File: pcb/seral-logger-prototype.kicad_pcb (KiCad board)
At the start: 2 copper layers, 108 x 23 mm, 49 parts, among them J1 Conn_ARM_JTAG_SWD_10, J2 Conn_01x04_Female, J3 Conn_01x04_Female, SW1 Rotary_Encoder_Switch_RGB, SW2 SW_SPST, U1 STM32G070KBT6, U2 74LVC3G17, U3 TLV70228_SOT23-5, U4 sn74lv1t34, U5 TLV61046ADB, U6 sn74lv1t34

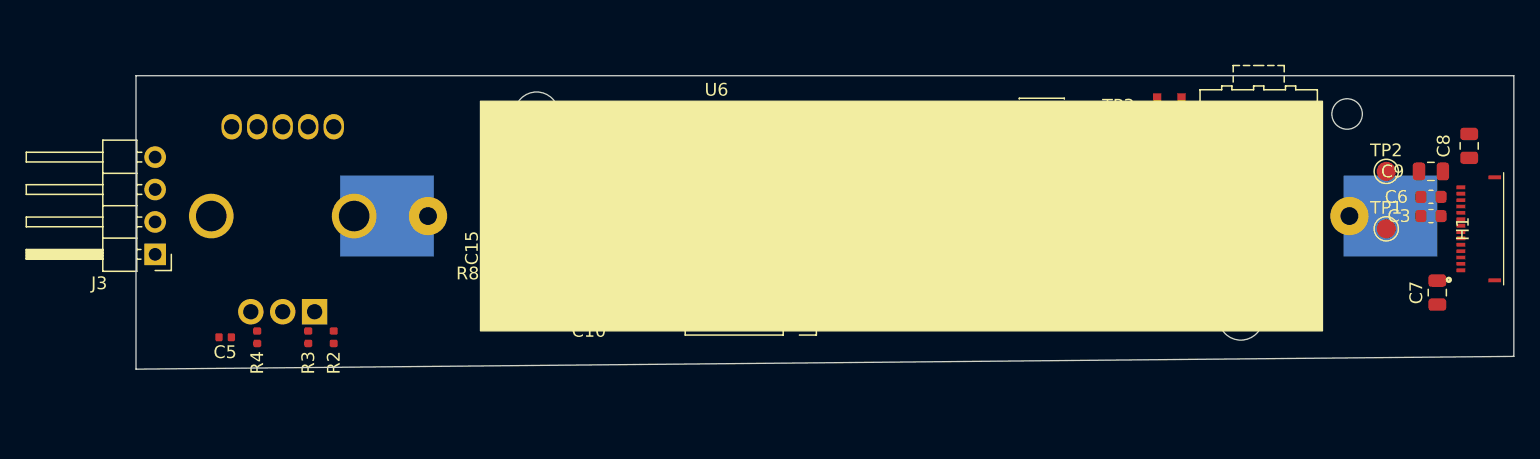
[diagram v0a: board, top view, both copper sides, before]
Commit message: Layout seems plausible: start routing
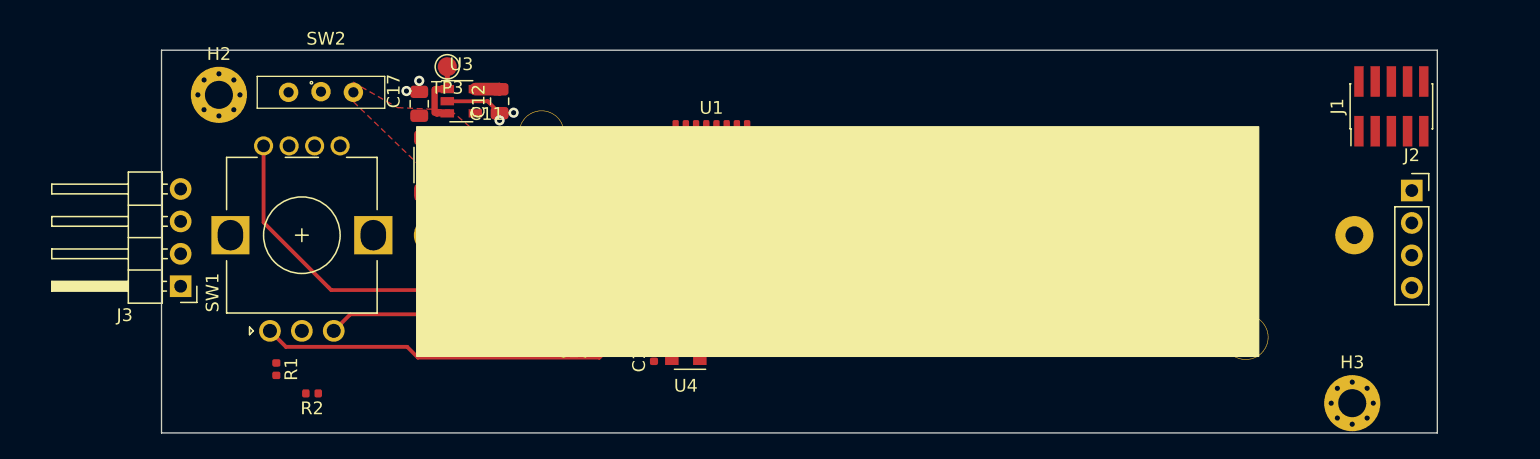
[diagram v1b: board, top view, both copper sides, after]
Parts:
- removed C5: 100nF, Capacitor_SMD:C_0402_1005Metric
- removed R3, R4: 220, Resistor_SMD:R_0402_1005Metric
- added H2: MountingHole_Pad, MountingHole:MountingHole_2.2mm_M2_Pad_Via, F.Cu at (26.5, 57.5)
- added H3: MountingHole_Pad, MountingHole:MountingHole_2.2mm_M2_Pad_Via, F.Cu at (115.3, 81.7)
- added R1: 220, Resistor_SMD:R_0402_1005Metric, F.Cu at (31.0, 79.0)
- BT1: footprint Jitter_Footprints:BatteryHolder_Keystone_1042(P)__1043(P)_1x18650 -> Jitter_Footprints:BatteryHolder_Keystone_1043(p)_1x18650
- R13, R5, R7: footprint Resistor_SMD:R_0402_1005Metric -> Resistor_SMD:R_0603_1608Metric
- SW1: value Rotary_Encoder_Switch_RGB -> Rotary_Encoder_Switch_DualLED; footprint Jitter_Footprints:Encoder_Switch_RGB_EC12PLRGBSDVBF -> Jitter_Footprints:PEL12D-4xxxS-Sxxxx; moved to F.Cu
- SW2: value SW_SPST -> SW_SPDT; footprint Button_Switch_SMD:SW_SPDT_CK-JS102011SAQN -> Jitter_Footprints:slide_switch_09.03201.02
- moved SW2 73.5 mm to (34.5, 57.3), turned to 0 degrees
- moved L1 67.1 mm to (43.5, 63.0), turned to 270 degrees
- moved C17 66.4 mm to (42.2, 58.2), turned to 270 degrees
- moved U5 59.0 mm to (47.5, 64.4), turned to 90 degrees
- moved U3 55.5 mm to (45.5, 58.0), turned to 0 degrees
- moved R14 55.5 mm to (48.0, 66.8), turned to 180 degrees
- moved C18 54.6 mm to (50.2, 64.4), turned to 90 degrees
- moved C11 54.6 mm to (47.5, 61.0), turned to 180 degrees
- moved R11 53.5 mm to (50.0, 66.8)
- moved TP3 52.8 mm to (44.4, 55.3), turned to 180 degrees
- moved C12 51.7 mm to (48.5, 58.0)
- moved TP4 50.6 mm to (53.0, 65.1), turned to 90 degrees
- moved J2 49.0 mm to (120.0, 65.0), turned to 0 degrees
- moved C3 42.0 mm to (79.5, 68.0)
- moved C6 42.0 mm to (79.5, 66.5)
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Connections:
- R12 pad 1: /SW -> /A
- R13 pad 1: GND -> /A
- R13 pad 2: /SW -> +3V3
- R5 pad 1: /A -> /B
- R6 pad 1: /A -> /B
- R7 pad 1: /B -> /SW
- R8 pad 1: /B -> /SW
- SW1 pad 1: Net-(R2-Pad2) -> GND
- SW1 pad 3: /SW -> Net-(R2-Pad2)
- SW1 pad 4: Net-(R4-Pad2) -> /SW
- U1 pad 21: /encoder_LED_B -> (no net)
- U2 pad 2: /encoder_B -> /encoder_BTN
- U2 pad 5: /encoder_BTN -> /encoder_A
- U2 pad 7: /encoder_A -> /encoder_B
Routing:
- net /A: track 0.00 -> 34.2 mm
- net /SW: track 0.00 -> 25.0 mm
- net /B: track 0.00 -> 24.8 mm
- net GND: track 0.00 -> 20.1 mm, vias 0 -> 13
- net +16V: track 0.00 -> 8.24 mm
- net +3V3: track 0.00 -> 6.61 mm
- net +BATT: track 0.00 -> 5.47 mm
- net Net-(C15-Pad1): track 0.00 -> 2.48 mm
- net Net-(C19-Pad1): track 0.00 -> 2.44 mm
- net Net-(C10-Pad1): track 0.00 -> 2.38 mm
- net Net-(R11-Pad2): track 0.00 -> 2.34 mm
- net /~NRST: track 0.00 -> 1.64 mm
- added copper zone on F.Cu, net +BATT
- added copper zone on F.Cu, net Net-(L1-Pad2)
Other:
- board size 108 x 23 mm -> 100 x 30 mm
